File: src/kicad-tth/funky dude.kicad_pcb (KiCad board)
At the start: 2 copper layers, 57.2 x 37.5 mm, 33 parts, among them P1 CONN_2, P2 CONN_2, P3 CONN_2, SW1 SWITCH_INV, SW2 SWITCH_INV, U1 OP284

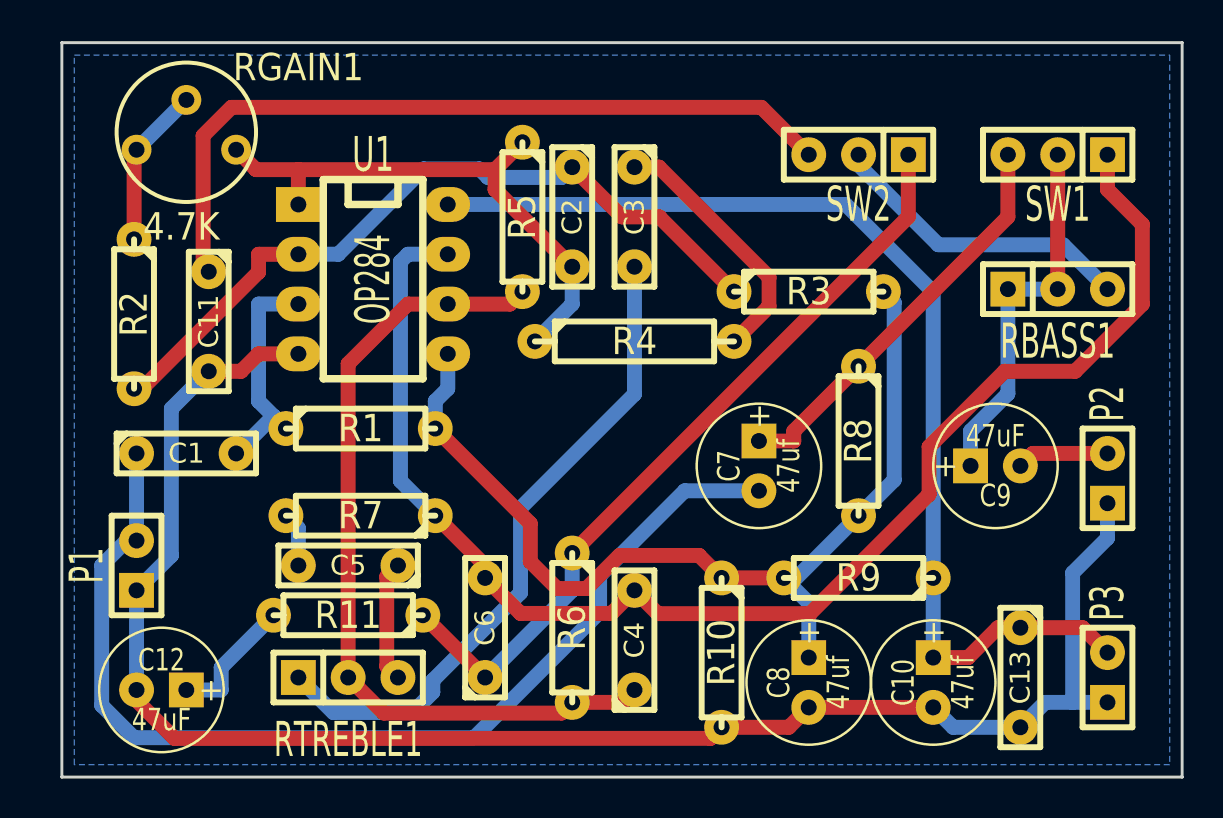
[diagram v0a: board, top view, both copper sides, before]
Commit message: 2014-10-22
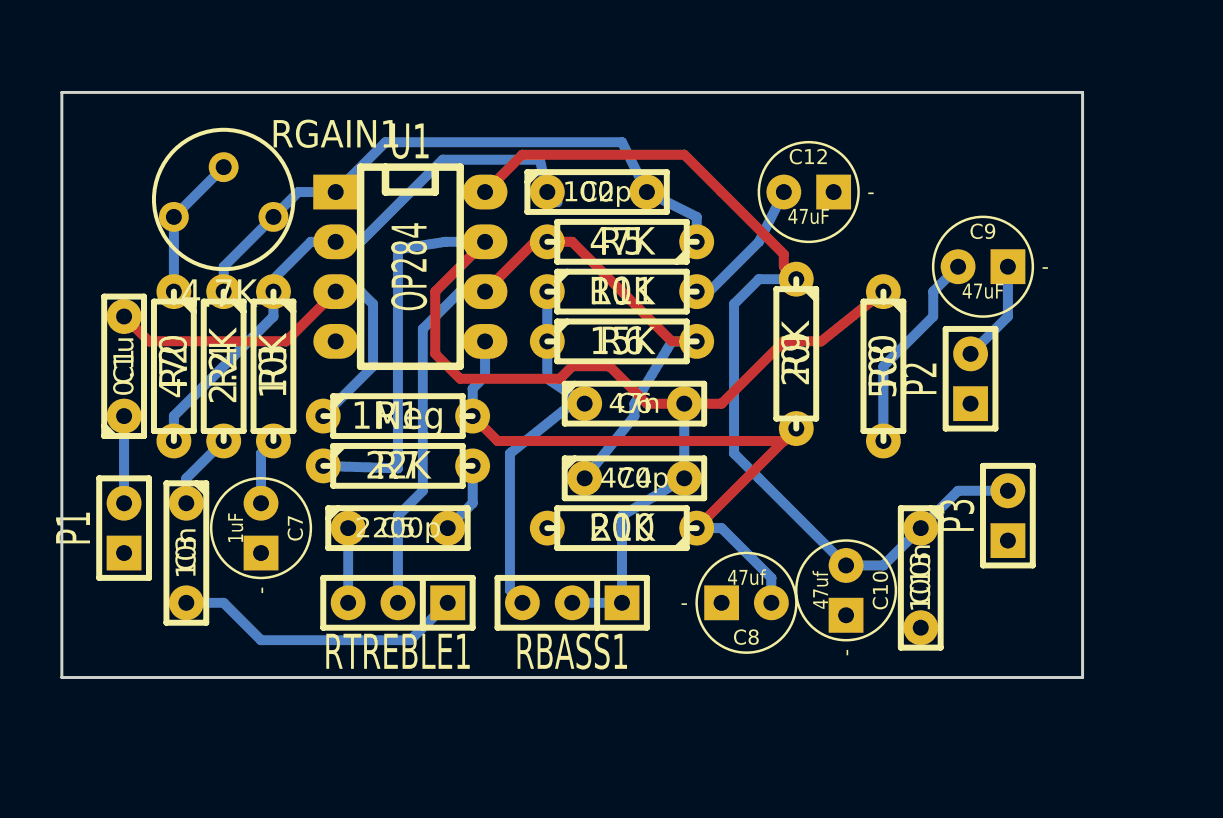
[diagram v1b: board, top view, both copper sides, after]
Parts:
- removed C11: 47nf, User:C2-LARGE_PADS
- removed SW1, SW2: SWITCH_INV, User:SIL-3-LARGE_PADS
- C1, C13, C2, C3, C4, C5, C6: footprint User:C2-LARGE_PADS -> Custom:C2-LARGE_PADS
- C10, C12, C8, C9: footprint User:C1V7-LARGE_PADS -> Custom:C1V5-LARGE_PADS
- C7: value 47uf -> 1uF; footprint User:C1V7-LARGE_PADS -> Custom:C1V5-LARGE_PADS
- P1, P2, P3: footprint User:SIL-2-LARGE_PADS -> Custom:SIL-2-LARGE_PADS
- R1, R10, R11, R2, R3, R5, R6, R7, R9: footprint User:R3-LARGE_PADS -> Custom:R3-LARGE_PADS
- R4: footprint User:R4-LARGE_PADS -> Custom:R3-LARGE_PADS
- R8: value 1Meg -> 500; footprint User:R3-LARGE_PADS -> Custom:R3-LARGE_PADS
- RBASS1, RTREBLE1: footprint User:SIL-3-LARGE_PADS -> Custom:SIL-3-LARGE_PADS
- U1: footprint User:DIP-8_LARGE_PADS -> Custom:DIP-8_LARGE_PADS
- moved C12 41.7 mm to (176.5, 111.8), turned to 0 degrees
- moved RBASS1 29.5 mm to (164.5, 132.7), turned to 180 degrees
- moved C3 28.6 mm to (144.8, 130.2)
- moved R3 27.6 mm to (149.2, 120.7), turned to 270 degrees
- moved C7 25.6 mm to (148.6, 128.9)
- moved R11 21.6 mm to (167.0, 116.8), turned to 0 degrees
- moved R4 21.0 mm to (146.7, 120.7), turned to 270 degrees
- moved R6 14.8 mm to (167.0, 119.4), turned to 0 degrees
- moved C6 13.7 mm to (167.6, 122.6), turned to 0 degrees
- moved R9 11.9 mm to (175.9, 120.0), turned to 270 degrees
- moved C9 10.2 mm to (185.4, 115.6)
- moved P3 9.69 mm to (186.7, 128.3)
- moved P2 8.64 mm to (184.8, 121.3)
- moved C4 8.26 mm to (167.6, 126.4), turned to 0 degrees
- moved R10 8.13 mm to (167.0, 128.9), turned to 180 degrees
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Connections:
- C7 pad 2: Net-(C1-Pad1) -> GND
- R3 pad 2: Vref -> Net-(C7-Pad1)
- R8 pad 1: Net-(C7-Pad1) -> Net-(C4-Pad2)
- R8 pad 2: Vref -> Net-(C9-Pad1)
- RBASS1 pad 1: Net-(C9-Pad1) -> Net-(C4-Pad2)
- RBASS1 pad 2: Net-(C9-Pad1) -> Net-(C4-Pad2)
- RBASS1 pad 3: Net-(RBASS1-Pad3) -> Net-(C6-Pad1)
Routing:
- net GND: track 86.1 -> 0.00 mm
- net Net-(C1-Pad1): track 54.4 -> 4.45 mm
- net Net-(C11-Pad1): track 39.5 -> 0.00 mm
- net Net-(C6-Pad1): track 40.1 -> 19.3 mm
- net Net-(C3-Pad2): track 34.0 -> 14.9 mm
- net Net-(C7-Pad1): track 20.9 -> 3.44 mm
- net Net-(RBASS1-Pad3): track 15.8 -> 0.00 mm
- net Vref: track 49.5 -> 35.1 mm
- net Net-(C2-Pad1): track 38.8 -> 28.9 mm
- net Net-(C1-Pad2): track 11.7 -> 21.3 mm
- net Net-(C3-Pad1): track 13.2 -> 3.96 mm
- net Net-(C9-Pad1): track 19.2 -> 10.5 mm
- net +9V: track 55.3 -> 48.9 mm
- net Net-(C4-Pad2): track 72.1 -> 67.4 mm
- net Net-(C2-Pad2): track 28.6 -> 31.2 mm
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- added copper zone on F.Cu, net GND
- removed copper zone on B.Cu, net GND
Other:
- board size 57.2 x 37.5 mm -> 52.1 x 29.8 mm
- net class Default: clearance 0.508 -> 0.381; trace_width 0.762 -> 0.508; via_dia 1.016 -> 0.762; via_drill 0.635 -> 0.508
- rule trace_clearance: 0.508 -> 0.381
- board text added: "V2.0-t"
- board text added: "funky dude preamp v2.0-t www.dolganoff.com"
- board text removed: "V1-t"
- board text removed: "funky dude preamp v1-t www.dolganoff.com"

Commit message: 2014-10-23
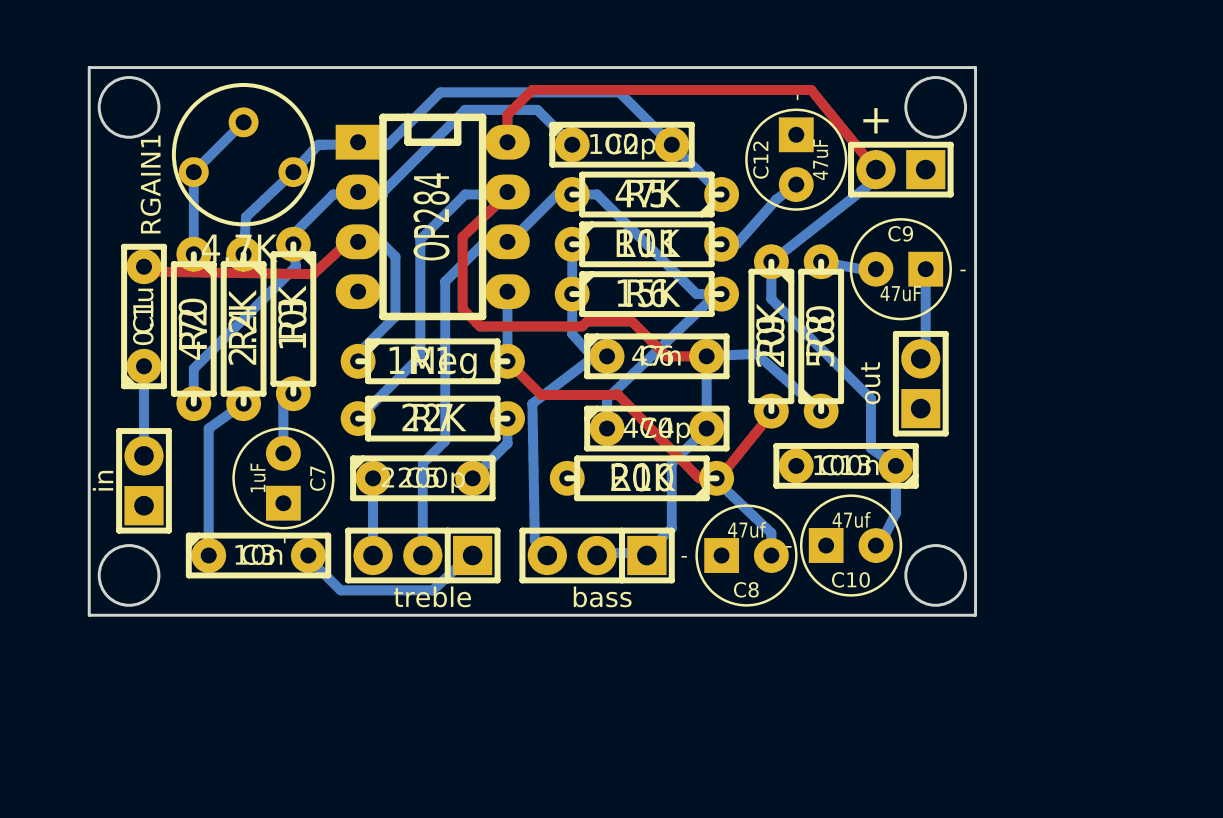
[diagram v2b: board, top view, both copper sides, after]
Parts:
- moved P3 18.5 mm to (181.2, 110.6), turned to 180 degrees
- moved C13 6.87 mm to (178.4, 125.7), turned to 180 degrees
- moved C9 4.19 mm to (181.2, 115.7)
- moved C3 3.69 mm to (148.5, 130.3), turned to 0 degrees
- moved R8 3.52 mm to (177.2, 119.1), turned to 90 degrees
- moved R1 3.31 mm to (157.4, 120.4)
- moved R7 3.00 mm to (157.4, 123.3)
- moved C5 2.84 mm to (156.8, 126.4)
- moved C7 2.79 mm to (149.7, 126.4)
- moved C4 2.79 mm to (168.8, 123.8)
- moved U1 2.79 mm to (157.4, 113.0)
- moved C1 2.74 mm to (142.6, 118.1)
- moved R10 2.74 mm to (168.0, 126.4)
- moved RBASS1 2.73 mm to (165.7, 130.3)
- moved RTREBLE1 2.73 mm to (156.8, 130.3)
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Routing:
- net Net-(C4-Pad2): track 67.4 -> 57.1 mm
- net Vref: track 35.1 -> 26.8 mm
- net Net-(C9-Pad1): track 10.5 -> 2.83 mm
- net Net-(C3-Pad2): track 14.9 -> 9.82 mm
- net Net-(C3-Pad1): track 3.96 -> 8.79 mm
- net Net-(C12-Pad1): track 7.07 -> 5.09 mm
- net +9V: track 48.9 -> 47.5 mm
- net Net-(C1-Pad2): track 21.3 -> 20.1 mm
- net Net-(C9-Pad2): track 5.23 -> 4.68 mm
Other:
- board size 52.1 x 29.8 mm -> 45.2 x 27.9 mm
- board text added: "+"
- board text added: "Licenced under CERN OHL v1.2"
- board text added: "Open Hardware"
- board text added: "bass"
- board text added: "in"
- board text added: "out"
- board text added: "treble"
- board text removed: "V2.0-t"

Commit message: 2014-10-23.2 - PCB is routed
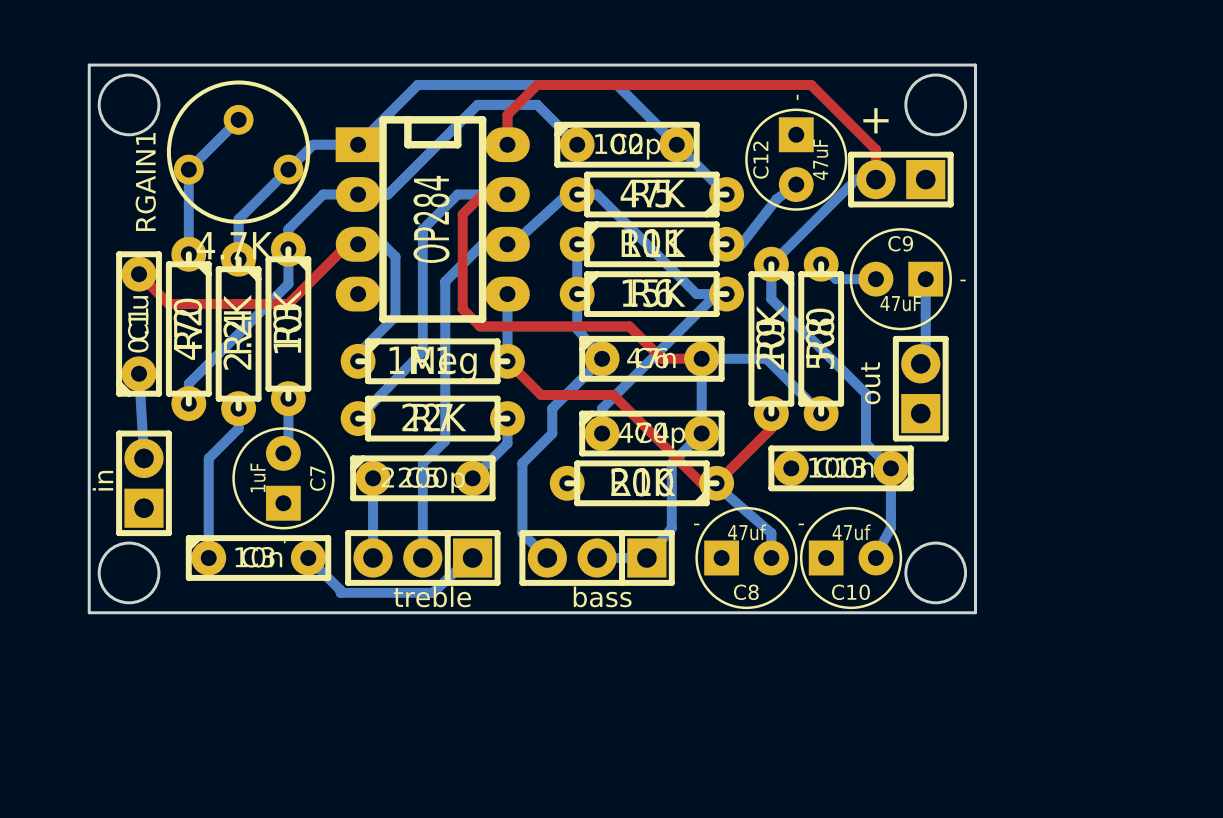
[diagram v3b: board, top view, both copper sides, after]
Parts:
- moved C10 0.63 mm to (178.7, 130.4)
- moved C9 0.51 mm to (181.2, 116.2)
- moved P3 0.51 mm to (181.2, 111.1)
- moved C1 0.46 mm to (142.4, 118.5)
- moved R3 0.36 mm to (150.0, 118.5)
- moved C4 0.36 mm to (168.5, 124.1)
- moved R4 0.36 mm to (147.4, 119.0)
- moved C6 0.28 mm to (168.5, 120.3)
- moved RGAIN1 0.28 mm to (147.4, 109.3)
- moved C13 0.28 mm to (178.2, 125.9)
- moved P2 0.25 mm to (182.2, 121.8)
- moved R10 0.25 mm to (168.0, 126.6)
- moved C2 0.25 mm to (167.3, 109.3)
- moved R11 0.25 mm to (168.5, 114.4)
- moved R2 0.25 mm to (144.9, 118.7)
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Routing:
- net Net-(C1-Pad2): track 20.1 -> 21.5 mm
- net Net-(C2-Pad2): track 31.0 -> 32.1 mm
- net +9V: track 47.5 -> 48.5 mm
- net Net-(C4-Pad1): track 41.9 -> 42.7 mm
- net Net-(C4-Pad2): track 57.1 -> 57.9 mm
- net Net-(C2-Pad1): track 28.5 -> 29.2 mm
- net Net-(C6-Pad1): track 19.4 -> 18.7 mm
- net Net-(C3-Pad1): track 8.79 -> 8.25 mm
